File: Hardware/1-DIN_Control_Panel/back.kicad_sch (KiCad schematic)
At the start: 49 parts, among them J1 Selector Knob Connector, J10 2x05 Molex Micro-Fit 3.0 43045, J13 Mode LEDs, J14 Selector Knob Connector, J15 Rotary Switch 1x7, J16 Mode LEDs, J2 Rotary Switch 1x7, J3 2x05 Molex Micro-Fit 3.0 43045, J4 UART Expansion, J5 SW - Aux Jump-Start, J6 SW - Battery Bypass, J7 SW - Master Power, J8 Pot/SW - Brightness, K1 FINDER-40.52, U12 LM324DR, U13 12V->5V Variable Boost Buck C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, U15 LTV-847S, U16 LTV-847S, U5 MMPQ3904, U6 MMPQ3904

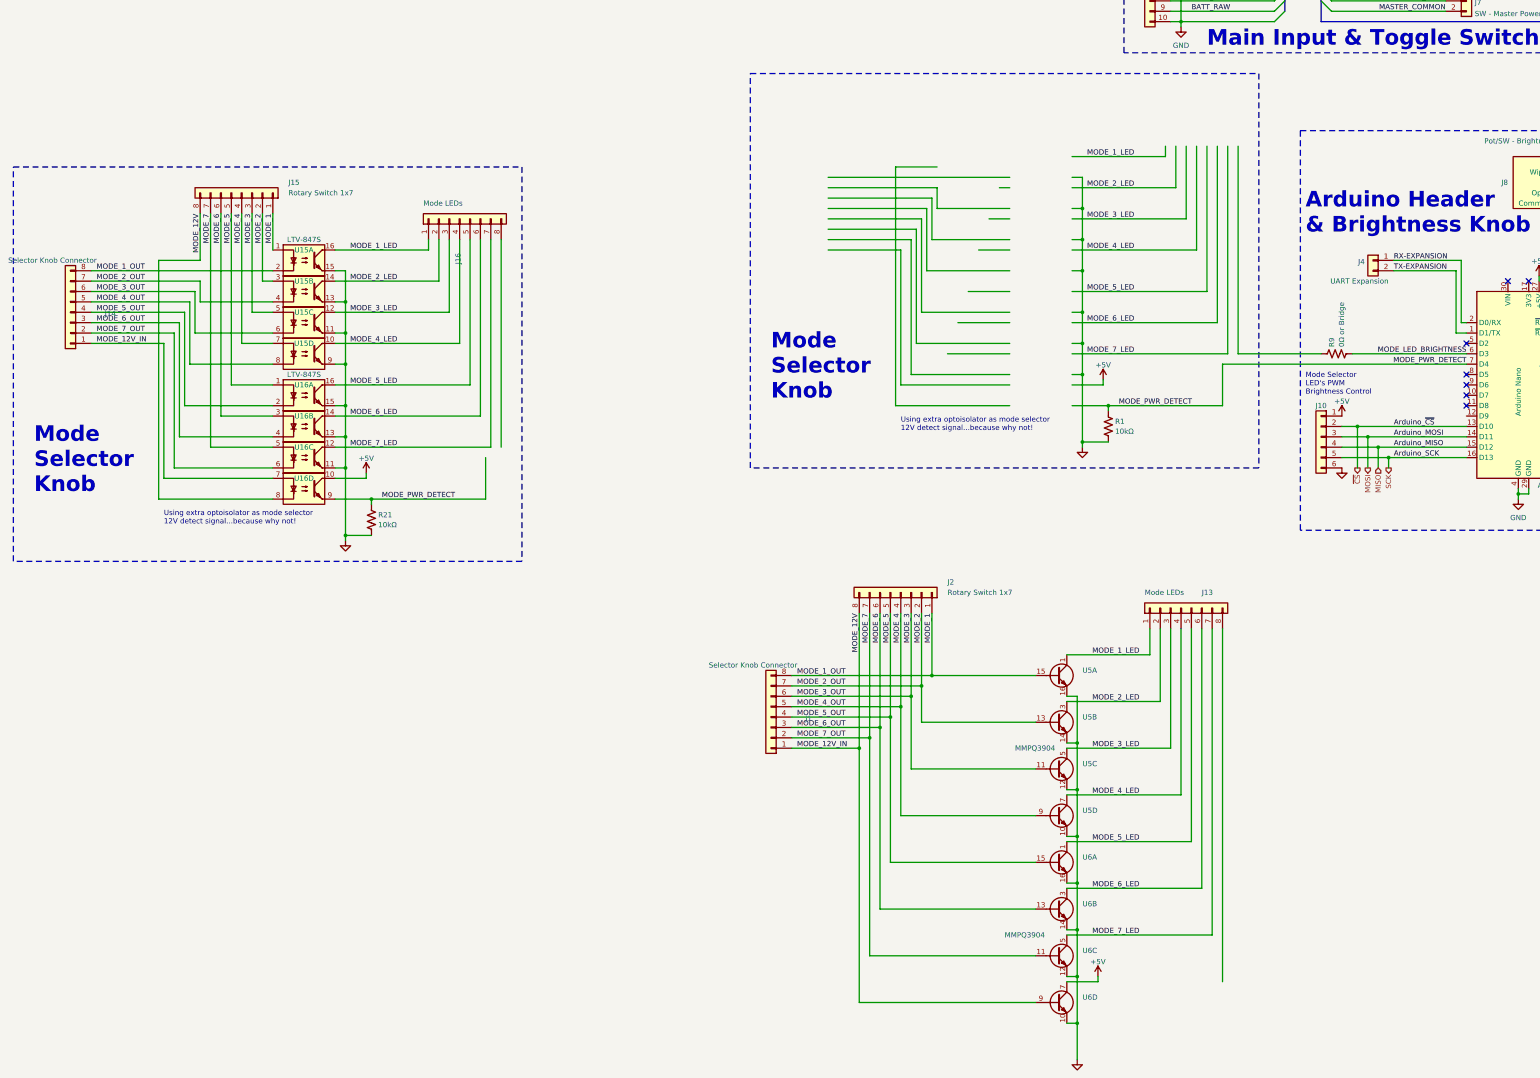
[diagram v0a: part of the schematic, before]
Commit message: Fixed BJT math
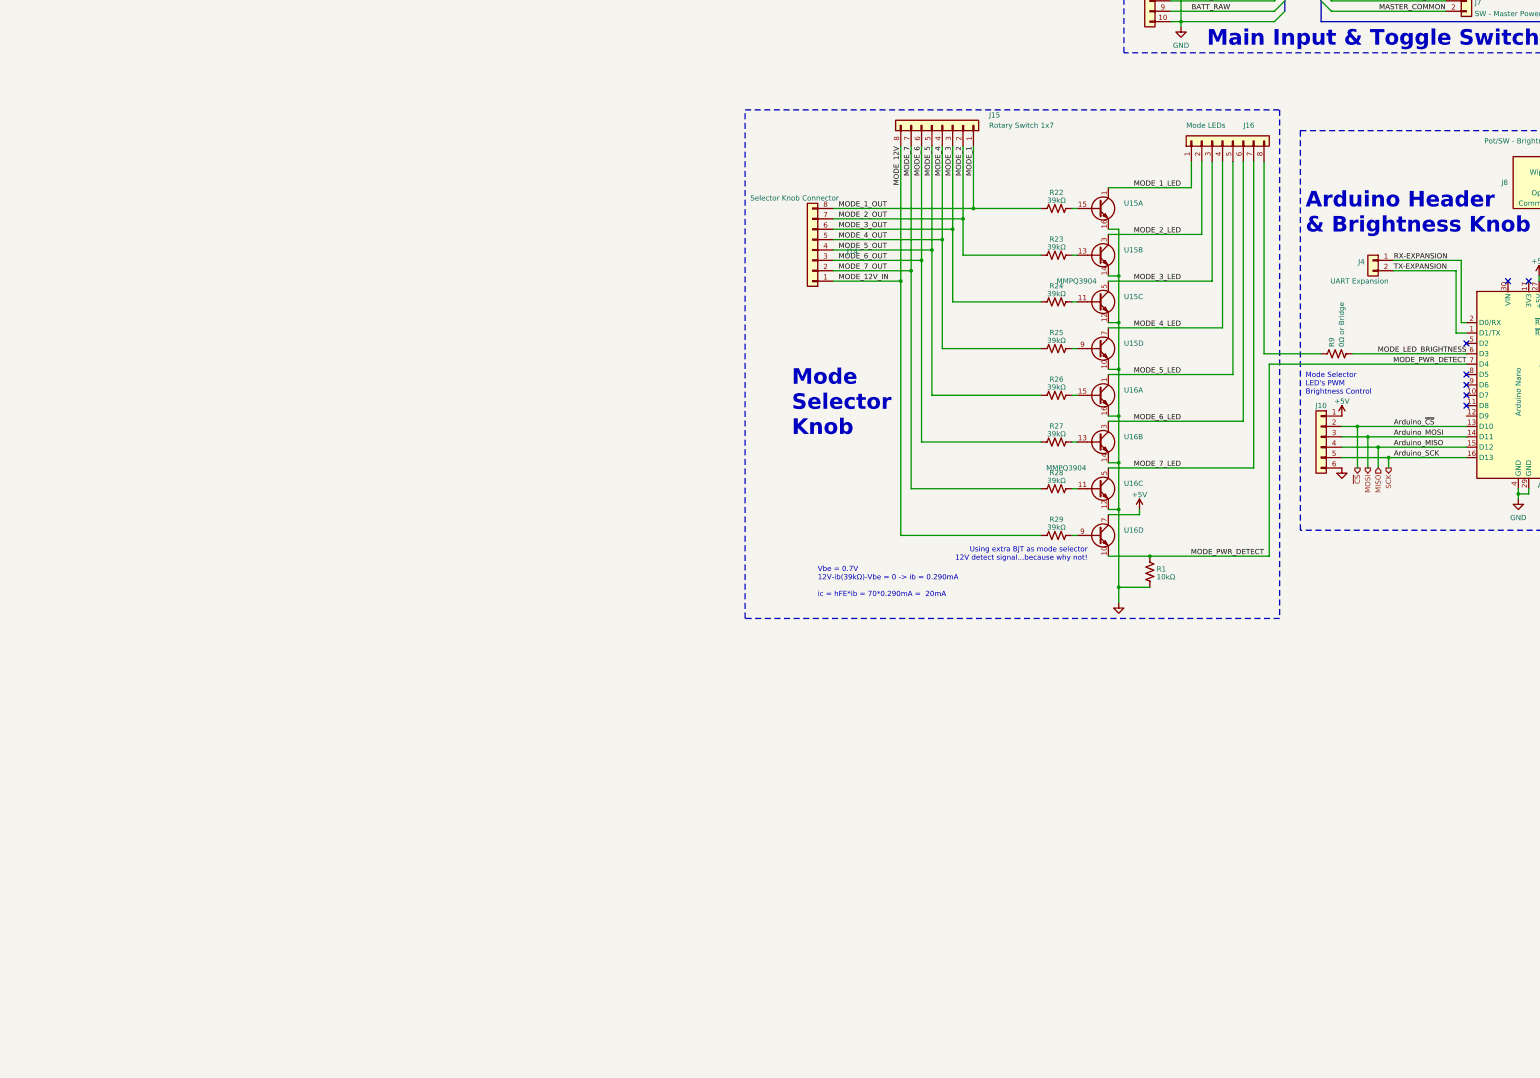
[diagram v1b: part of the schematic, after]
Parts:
- removed J14: Selector Knob Connector, Connector_Molex:Molex_Micro-Fit_3.0_43045-0812_2x04_P3.00mm_Vertical, symbol Connector_Generic:Conn_01x08
- removed J15: Rotary Switch 1x7, Connector_Molex:Molex_Micro-Fit_3.0_43045-0812_2x04_P3.00mm_Vertical, symbol Connector_Generic:Conn_01x08
- removed J16: Mode LEDs, Connector_Molex:Molex_Micro-Fit_3.0_43045-0812_2x04_P3.00mm_Vertical, symbol Connector_Generic:Conn_01x08
- removed R21: 10kΩ, Resistor_SMD:R_0603_1608Metric_Pad0.98x0.95mm_HandSolder, symbol Device:R_US
- removed U15, U16: LTV-847S, Package_DIP:SMDIP-16_W9.53mm, symbol Isolator:LTV-847S
- added R22, R23, R24, R25, R26, R27, R28, R29: 39kΩ, Resistor_SMD:R_0603_1608Metric_Pad0.98x0.95mm_HandSolder, symbol Device:R_US
- renumbered J1 to J14, J2 to J15, J13 to J16, U5 to U15, U6 to U16
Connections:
- net GND: no longer U16.10 (E4)
- net MODE_1: now also R22.2; no longer U15.15 (B1)
- net MODE_12V: now also R29.2; no longer U16.9 (B4)
- net MODE_2: now also R23.2; no longer U15.13 (B2)
- net MODE_3: now also R24.2; no longer U15.11 (B3)
- net MODE_4: now also R25.2; no longer U15.9 (B4)
- net MODE_5: now also R26.2; no longer U16.15 (B1)
- net MODE_6: now also R27.2; no longer U16.13 (B2)
- net MODE_7: now also R28.2; no longer U16.11 (B3)
- net MODE_PWR_DETECT: now also U16.10 (E4)
- net at J16.8 (Pin_8): now also R9.2
- new net: R27.1, U16.13 (B2)
- new net: R24.1, U15.11 (B3)
- new net: R23.1, U15.13 (B2)
- new net: R26.1, U16.15 (B1)
- new net: R25.1, U15.9 (B4)
- new net: R22.1, U15.15 (B1)
- new net: R28.1, U16.11 (B3)
- new net: R29.1, U16.9 (B4)
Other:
- note added: "Using extra BJT as mode selector 12V detect signal...because why not!"
- note added: "Vbe = 0.7V 12V-ib(39kΩ)-Vbe = 0 -> ib = 0.290mA ic = hFE*ib = 70*0.290mA = 20mA"
- note removed: "Using extra optoisolator as mode selector 12V detect signal...because why not!"
- moved on the sheet: J14, J15, J16, U15A, U15B, U15C, U15D, U16A, U16B, U16C, U16D
